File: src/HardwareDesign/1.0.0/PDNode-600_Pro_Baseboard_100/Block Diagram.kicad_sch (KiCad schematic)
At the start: 0 parts

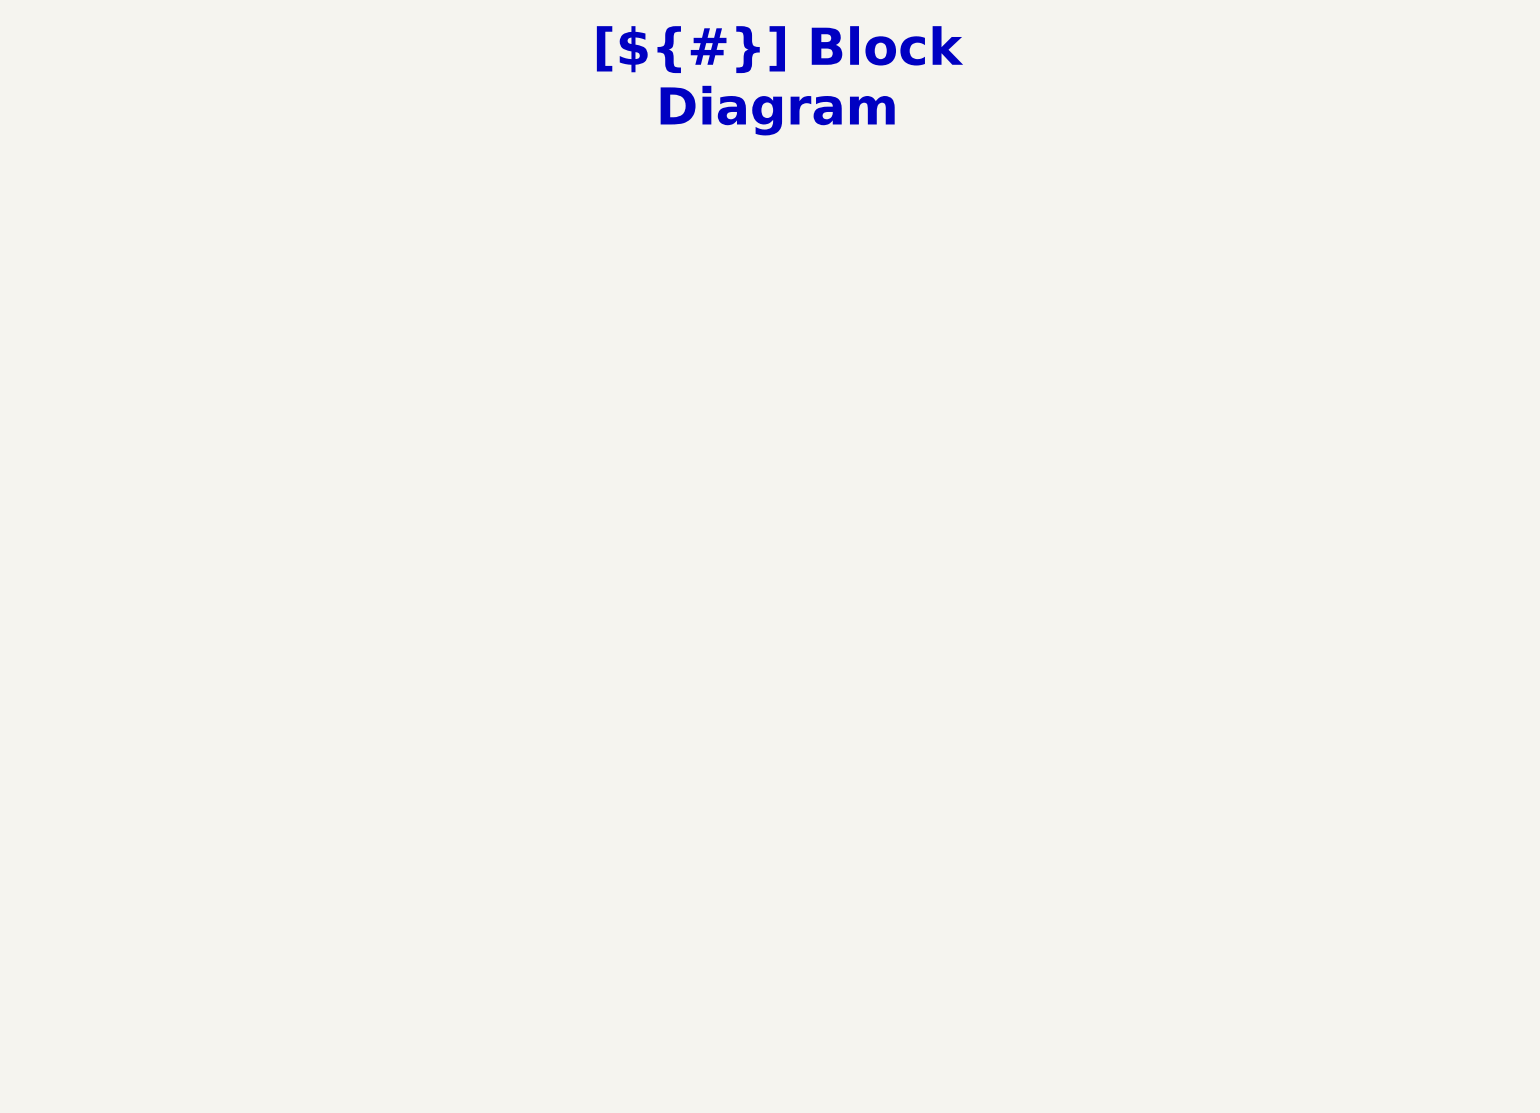
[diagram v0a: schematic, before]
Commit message: update readme, add documentation
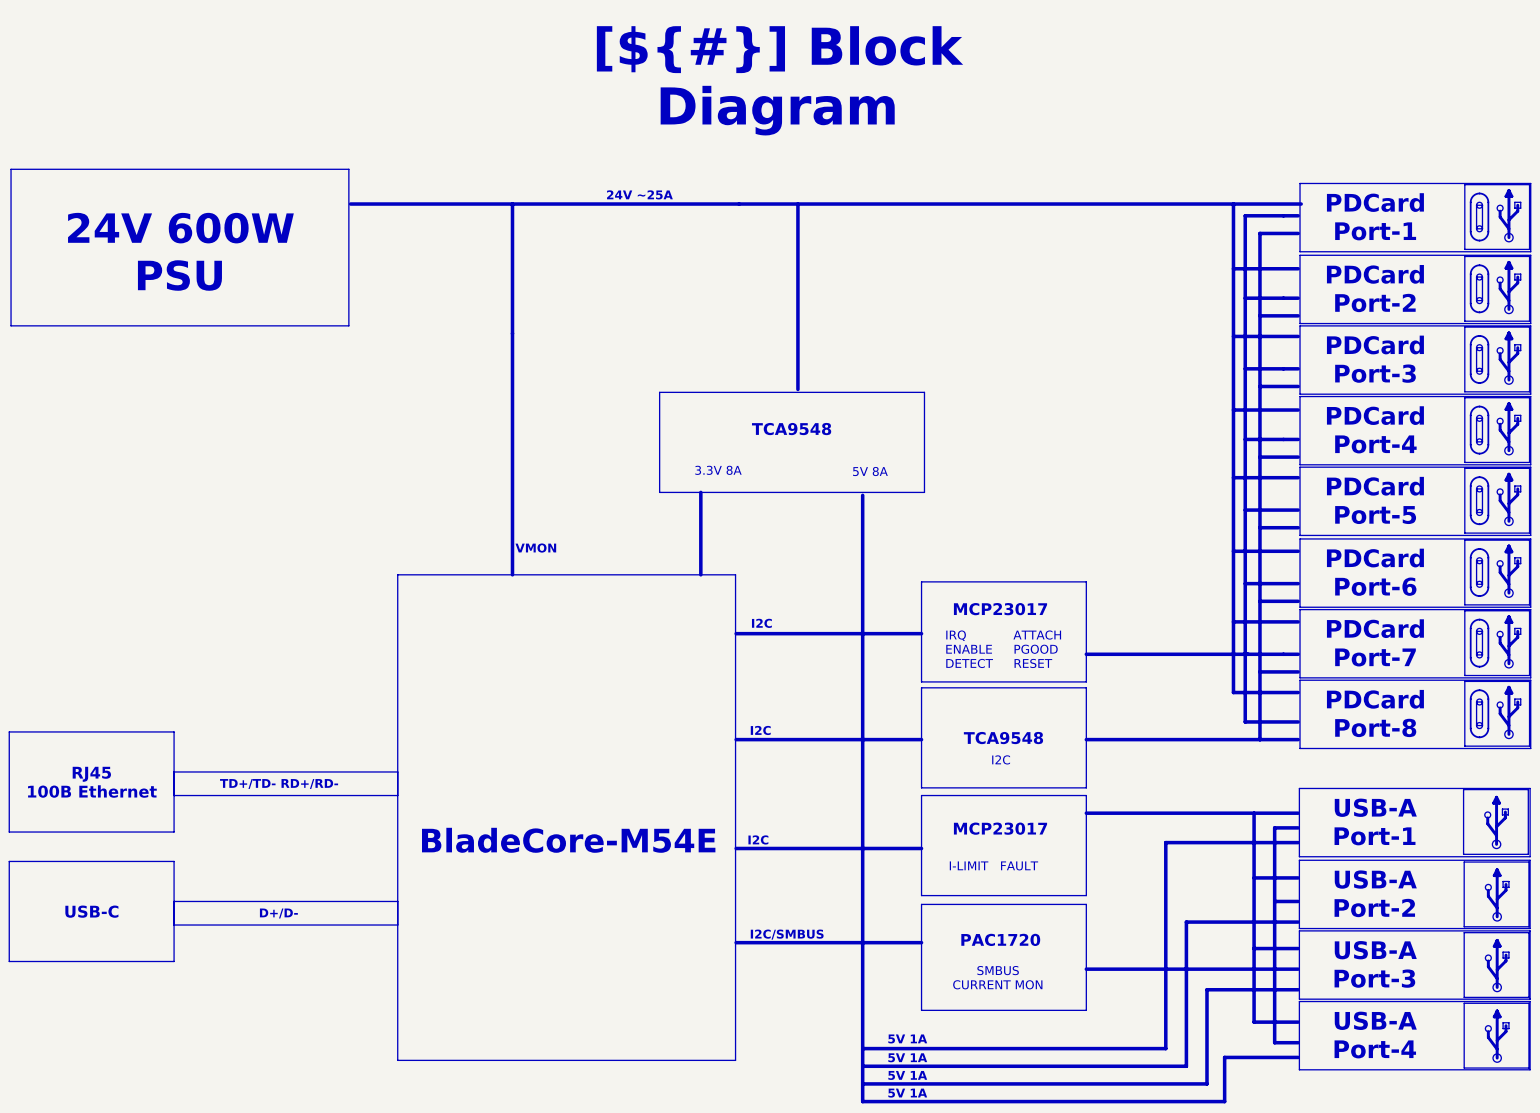
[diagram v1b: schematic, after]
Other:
- note added: "24V 600W PSU"
- note added: "24V ~25A"
- note added: "3.3V 8A"
- note added: "5V 1A"
- note added: "5V 8A"
- note added: "ATTACH PGOOD RESET"
- note added: "BladeCore-M54E"
- note added: "D+/D-"
- note added: "I-LIMIT FAULT"
- note added: "I2C"
- note added: "I2C/SMBUS"
- note added: "IRQ ENABLE DETECT"
- note added: "MCP23017"
- note added: "PAC1720"
- note added: "PDCard Port-1"
- note added: "PDCard Port-2"
- note added: "PDCard Port-3"
- note added: "PDCard Port-4"
- note added: "PDCard Port-5"
- note added: "PDCard Port-6"
- note added: "PDCard Port-7"
- note added: "PDCard Port-8"
- note added: "RJ45 100B Ethernet"
- note added: "SMBUS CURRENT MON"
- note added: "TCA9548"
- note added: "TD+/TD- RD+/RD-"
- note added: "USB-A Port-1"
- note added: "USB-A Port-2"
- note added: "USB-A Port-3"
- note added: "USB-A Port-4"
- note added: "USB-C"
- note added: "VMON"
